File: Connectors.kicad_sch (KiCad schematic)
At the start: 13 parts

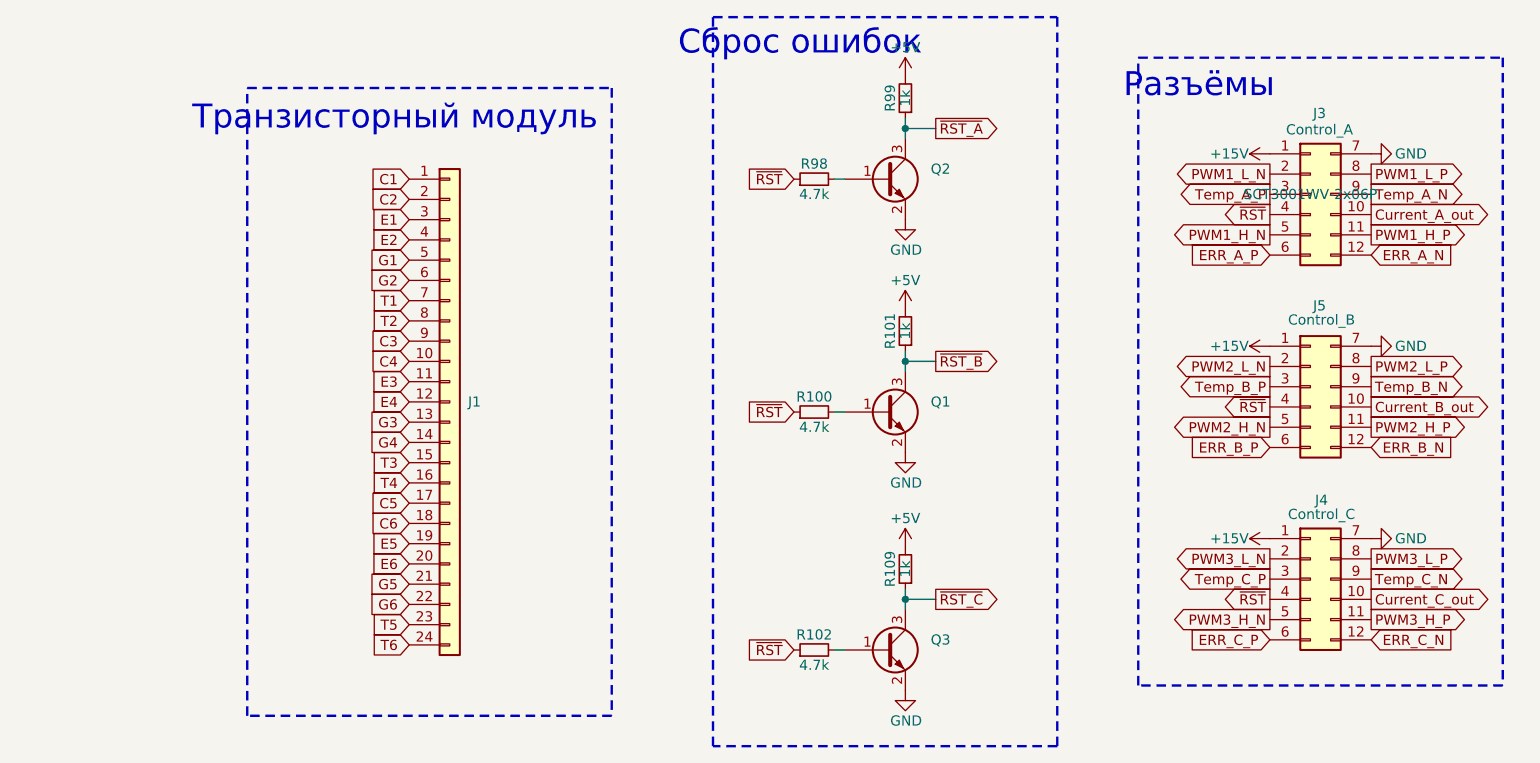
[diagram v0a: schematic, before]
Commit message: VER2.2.1: создал папку для производственных доков
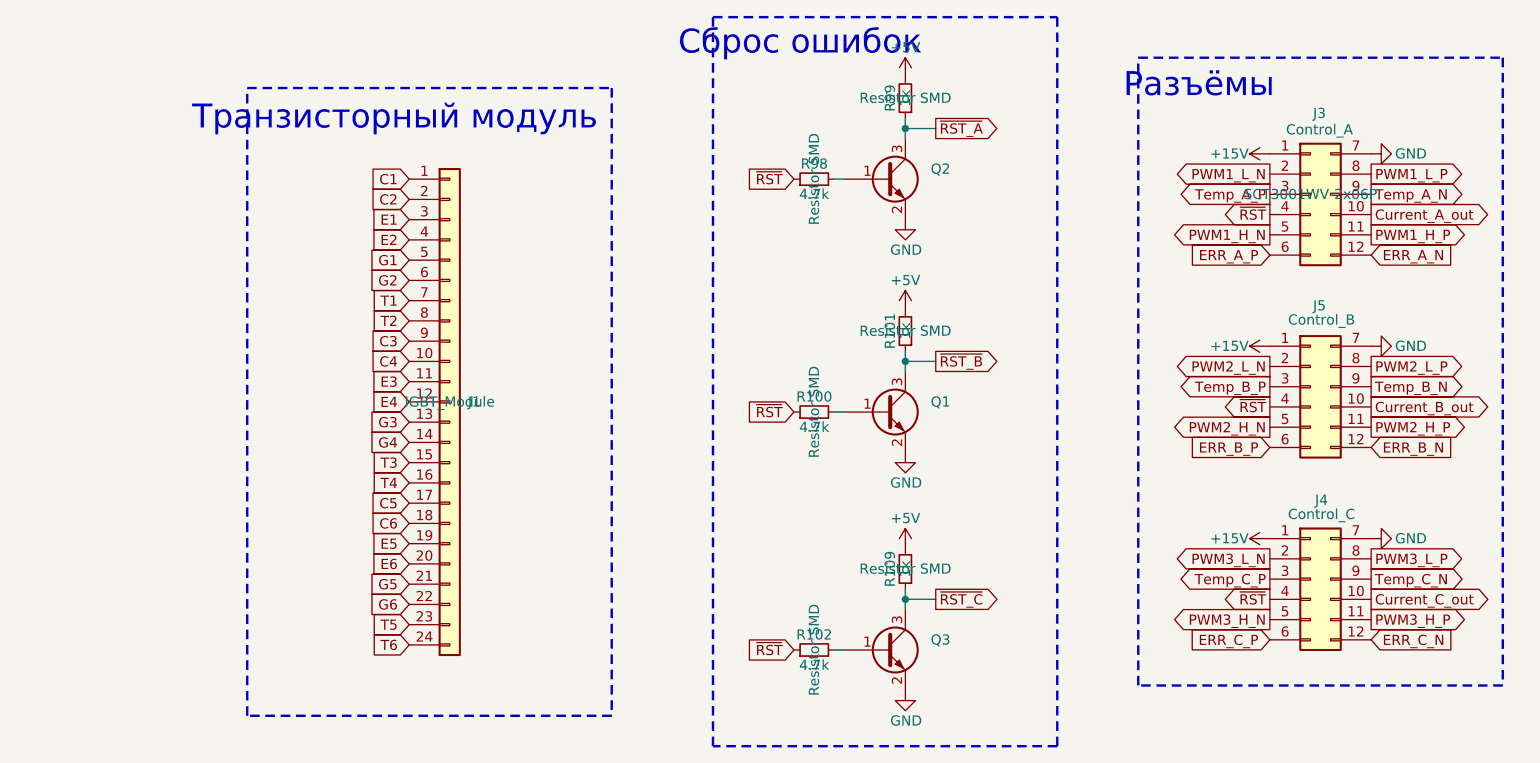
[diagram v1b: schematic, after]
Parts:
- J1: Description P/N (none) -> IGBT_Module
- R100, R101, R102, R109, R98, R99: Description P/N (none) -> Resistor SMD
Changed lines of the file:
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@@
 			)
 		)
-		(property "Description P/N" ""
+		(property "Description P/N" "Resistor SMD"
 			(at 157.48 60.96 0)
 			(effects
@@
 			)
 		)
-		(property "Description P/N" ""
+		(property "Description P/N" "Resistor SMD"
 			(at 146.05 130.175 0)
 			(effects
@@
 			)
 		)
-		(property "Description P/N" ""
+		(property "Description P/N" "Resistor SMD"
 			(at 146.05 100.33 0)
 			(effects
@@
 			)
 		)
-		(property "Description P/N" ""
+		(property "Description P/N" "Resistor SMD"
 			(at 157.48 90.17 0)
 			(effects
@@
 			)
 		)
-		(property "Description P/N" ""
+		(property "Description P/N" "Resistor SMD"
 			(at 146.05 71.12 0)
 			(effects
@@
 			)
 		)
-		(property "Description P/N" ""
+		(property "Description P/N" "Resistor SMD"
 			(at 157.48 120.015 0)
 			(effects
@@
 			)
 		)
-		(property "Description P/N" ""
+		(property "Description P/N" "IGBT_Module"
 			(at 100.33 99.06 0)
 			(effects

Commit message: VER2.2.1: исправил все доки
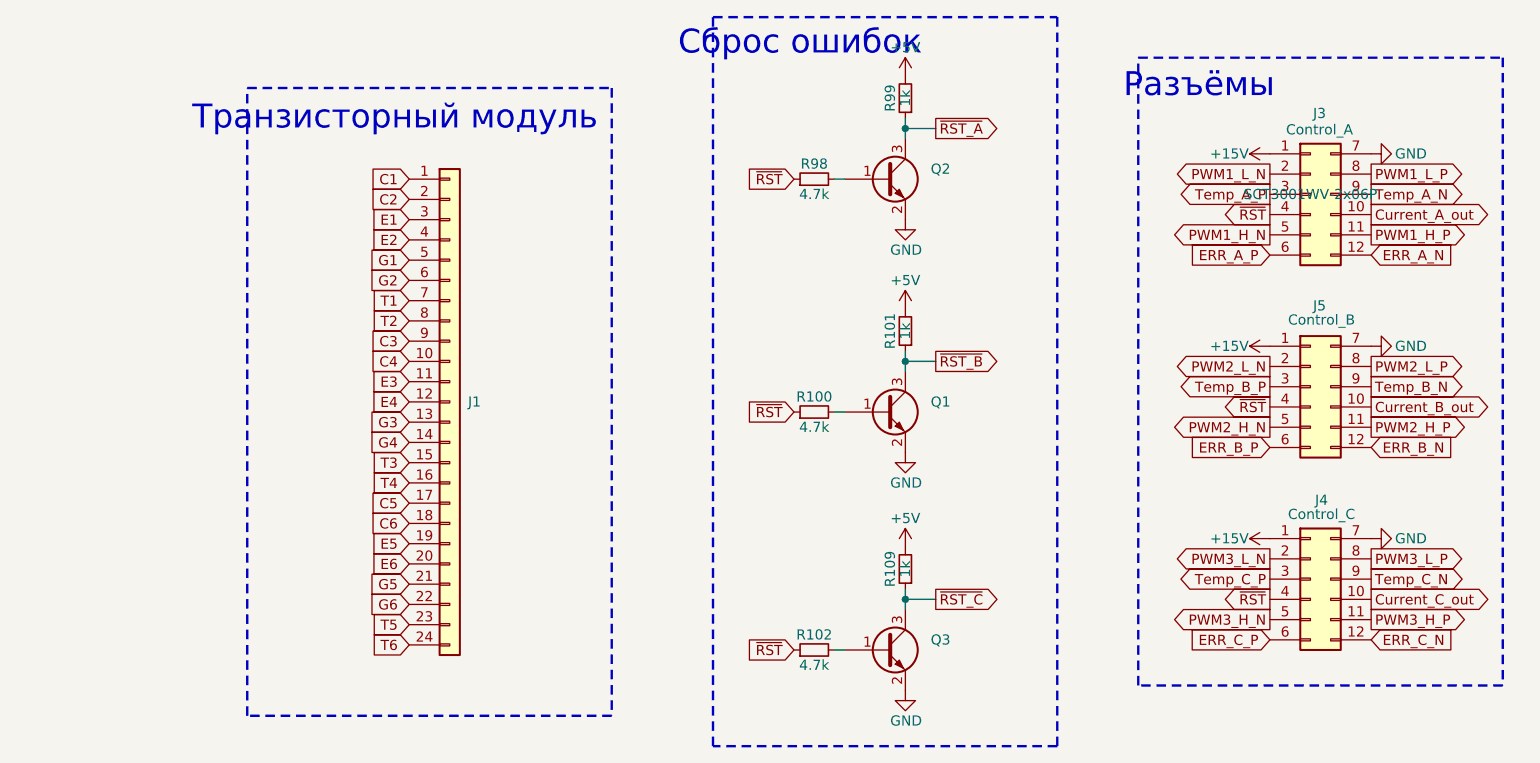
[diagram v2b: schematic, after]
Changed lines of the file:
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@@
 		(date "2025-06-04")
 		(company "ООО \"ЭТТ\"")
+		(comment 1 "НВЦТ.EVP150-2-1.2000.120_v1 Э3")
 	)
 	(rectangle
@@
 					(size 1.27 1.27)
 				)
+				(hide yes)
 			)
 		)
@@
 					(size 1.27 1.27)
 				)
+				(hide yes)
 			)
 		)
@@
 					(size 1.27 1.27)
 				)
+				(hide yes)
 			)
 		)
@@
 					(size 1.27 1.27)
 				)
+				(hide yes)
 			)
 		)
@@
 					(size 1.27 1.27)
 				)
+				(hide yes)
 			)
 		)
@@
 					(size 1.27 1.27)
 				)
+				(hide yes)
 			)
 		)
@@
 					(size 1.27 1.27)
 				)
+				(hide yes)
 			)
 		)
